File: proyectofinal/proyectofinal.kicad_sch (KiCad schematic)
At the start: 13 parts, among them J1 cnn, J2 conector paramodulo lora, J3 dht22, J4 Guva-s12s, J5 convertidor_TTL, U1 LM7833_TO220, U2 ESP32_DevKit_V1_DOIT, U3 LM7805_TO220

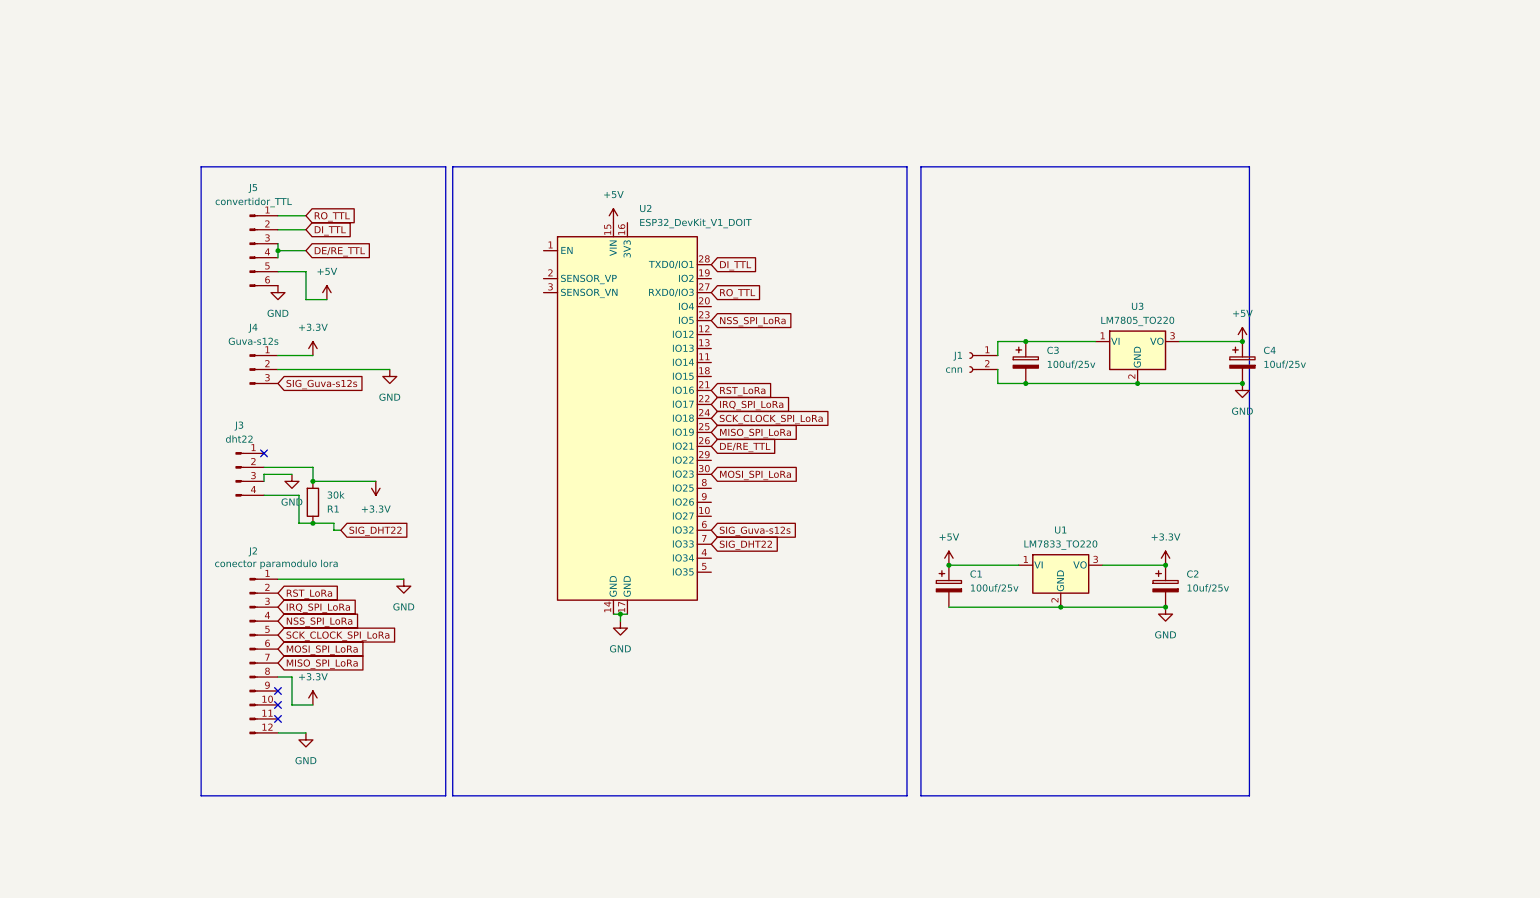
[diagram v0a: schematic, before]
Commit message: e
e
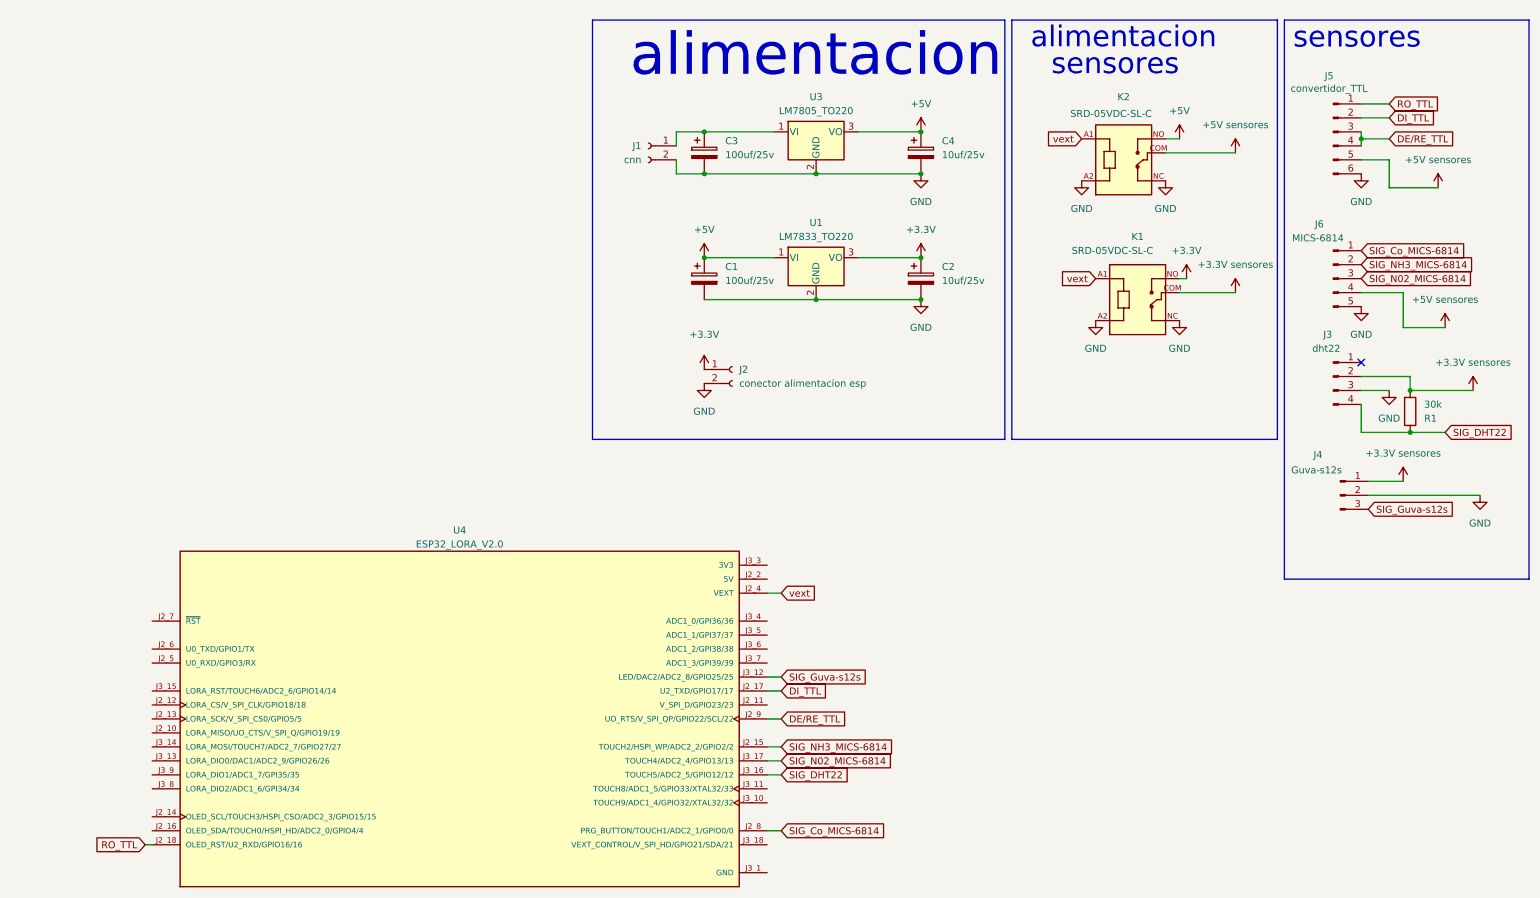
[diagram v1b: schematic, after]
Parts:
- removed J2: conector paramodulo lora, Connector_Molex:Molex_SL_171971-0012_1x12_P2.54mm_Vertical, symbol Connector:Conn_01x12_Pin
- removed U2: ESP32_DevKit_V1_DOIT, esp32_devkit_v1_doit:esp32_devkit_v1_doit, symbol esp32_devkit_v1_doit:ESP32_DevKit_V1_DOIT
- added J2: conector alimentacion esp, Connector_JST:JST_EH_B2B-EH-A_1x02_P2.50mm_Vertical, symbol Connector:Conn_01x02_Socket
- added J6: MICS-6814, Connector_Molex:Molex_KK-254_AE-6410-05A_1x05_P2.54mm_Vertical, symbol Connector:Conn_01x05_Pin
- added K1, K2: SRD-05VDC-SL-C, SRD-05VDC-SL-C:RELAY_SRD-05VDC-SL-C, symbol SRD-05VDC-SL-C:SRD-05VDC-SL-C
- added U4: ESP32_LORA_V2.0, ESP32_LORA_V2.0:MODULE_ESP32_LORA_V2.0, symbol ESP32_LORA_V2.0:ESP32_LORA_V2.0
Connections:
- net +3.3V: now also J2.1 (Pin_1), K1.NO; no longer J3.2 (Pin_2), J4.1 (Pin_1), R1.2
- net +5V: now also K2.NO; no longer J5.5 (Pin_5)
- net DE/RE_TTL: now also U4.J2_9 (UO_RTS/V_SPI_QP/GPIO22/SCL/22)
- net DI_TTL: now also U4.J2_17 (U2_TXD/GPIO17/17)
- net GND: now also J2.2 (Pin_2), J6.5 (Pin_5), K1.A2, K1.NC, K2.A2, K2.NC
- net RO_TTL: now also U4.J2_18 (OLED_RST/U2_RXD/GPIO16/16)
- net SIG_DHT22: now also U4.J3_16 (TOUCH5/ADC2_5/GPIO12/12)
- net SIG_Guva-s12s: now also U4.J3_12 (LED/DAC2/ADC2_8/GPIO25/25)
- new net: U4. (GND), U4.J3_1 (GND)
- new net: U4. (GND), U4.J3_3 (3V3)
- new net +3.3V sensores: J3.2 (Pin_2), J4.1 (Pin_1), K1.COM, R1.2
- new net +5V sensores: J5.5 (Pin_5), J6.4 (Pin_4), K2.COM
- new net SIG_Co_MICS-6814: J6.1 (Pin_1), U4.J2_8 (PRG_BUTTON/TOUCH1/ADC2_1/GPIO0/0)
- new net SIG_N02_MICS-6814: J6.3 (Pin_3), U4.J3_17 (TOUCH4/ADC2_4/GPIO13/13)
- new net SIG_NH3_MICS-6814: J6.2 (Pin_2), U4.J2_15 (TOUCH2/HSPI_WP/ADC2_2/GPIO2/2)
- new net vext: K1.A1, K2.A1, U4. (GND), U4.J2_4 (VEXT)
- no-connect marks 4 -> 1
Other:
- note added: "alimentacion"
- note added: "sensores"
- moved on the sheet: C1, C2, C3, C4, J1, J3, J4, J5, R1, U1, U3

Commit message: w
w
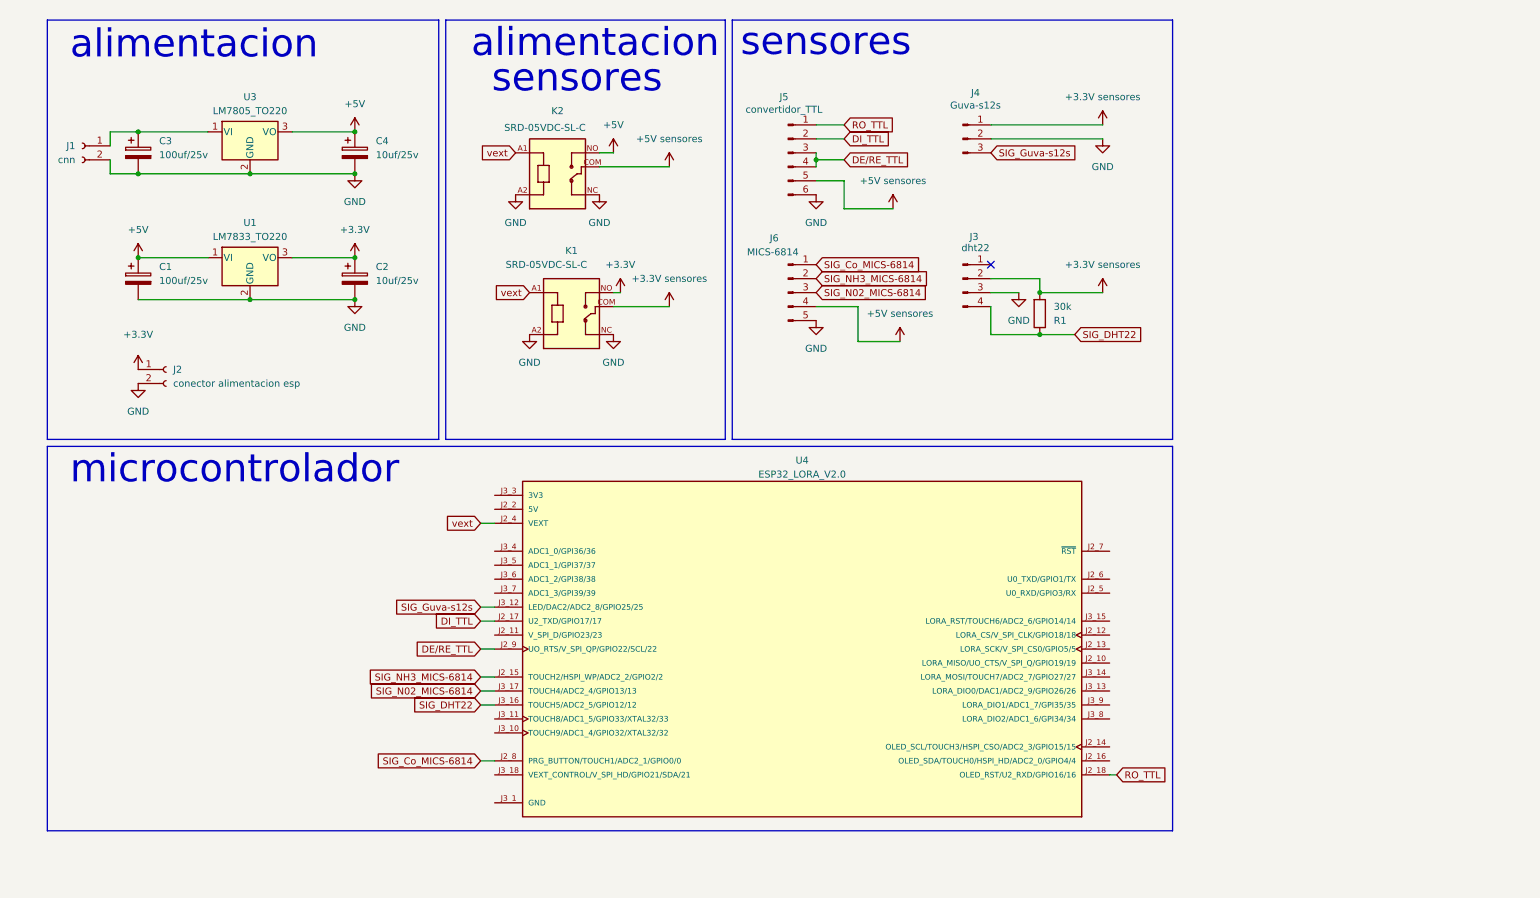
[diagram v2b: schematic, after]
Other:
- note added: "microcontrolador"
- moved on the sheet: C1, C2, C3, C4, J1, J2, J3, J4, J5, J6, K1, K2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
